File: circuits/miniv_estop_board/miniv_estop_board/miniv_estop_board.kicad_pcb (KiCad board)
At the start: 2 copper layers, 100 x 130 mm, 47 parts, among them J1 Conn_Main_DCDC, J2 Conn_neopixel_01, J3 Conn_neopixel_02, J4 Conn_neopixel_03, J5 Conn_neopixel_04, J6 EStop_button, J7 EStop_signal0, J8 EStop_signal1, Q1 2SJ555-E, Q2 NPN, Q3 NPN, Q4 NPN, Q6 2SJ555-E, Q7 NPN, U1 Teensy4.1

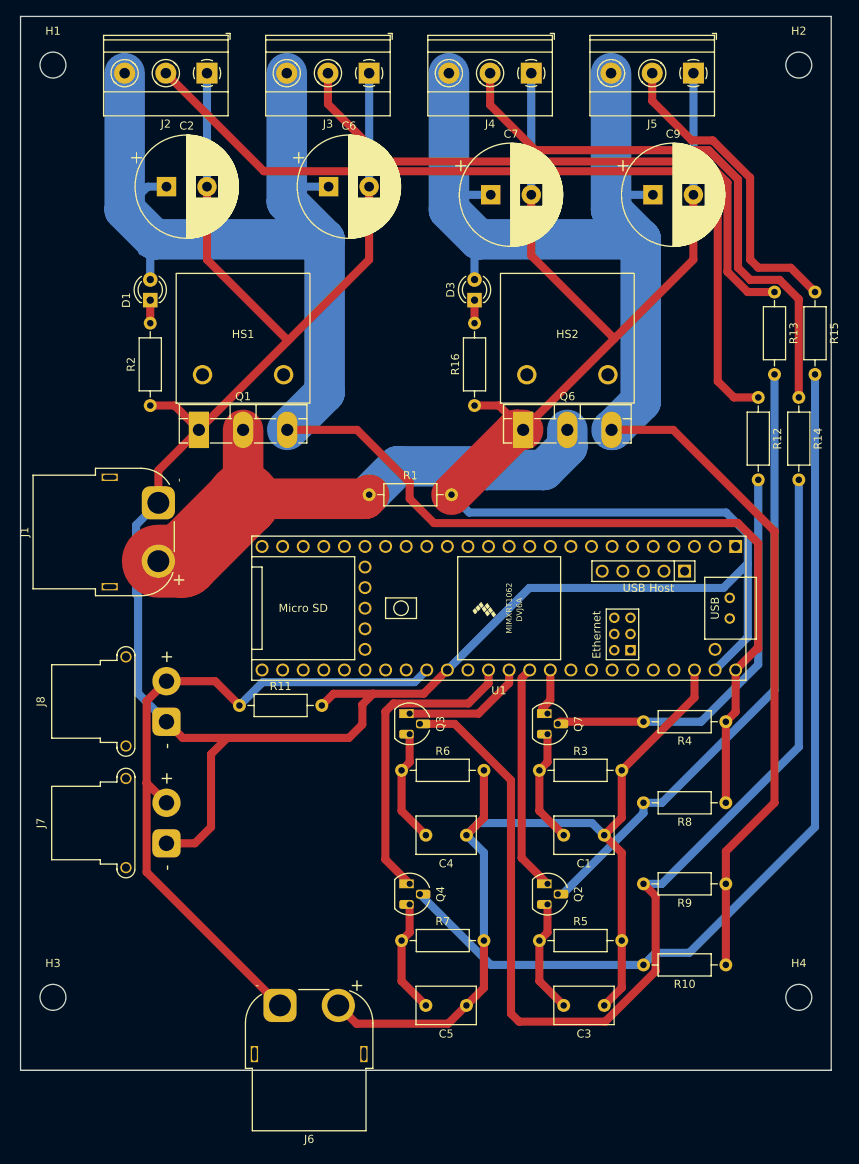
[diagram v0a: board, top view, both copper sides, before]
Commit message: update pcb
Signed-off-by: Masaya Kataoka <ms.kataoka@gmail.com>
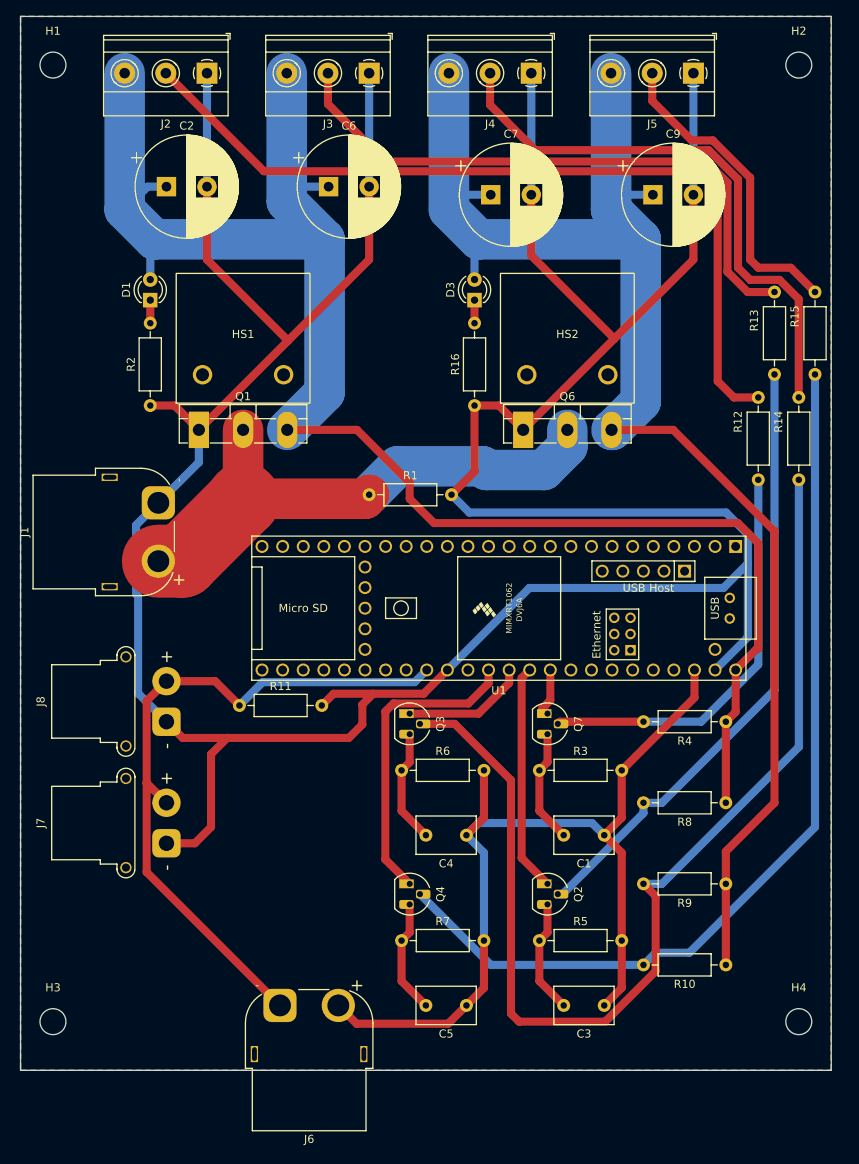
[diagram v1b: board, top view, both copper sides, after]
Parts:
- moved H3 3.00 mm to (96.0, 137.0)
- moved H4 3.00 mm to (188.0, 137.0)
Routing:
- net Net-(D1-A): track 209.2 -> 207.1 mm
- added copper zone on B.Cu, net GND
- added copper zone on F.Cu, net GND
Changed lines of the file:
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@@
 			(layer "F.Fab")
 		)
-		(fp_text user "-"
-			(at 2.8 2.5 90)
+		(fp_text user "+"
+			(at -9.5 2.5 90)
 			(layer "F.SilkS")
 			(effects
 				(font
-					(size 1 1)
+					(size 1.5 1.5)
 					(thickness 0.15)
 				)
 			)
 		)
-		(fp_text user "+"
-			(at -9.5 2.5 90)
+		(fp_text user "-"
+			(at 2.8 2.5 90)
 			(layer "F.SilkS")
 			(effects
 				(font
-					(size 1.5 1.5)
+					(size 1 1)
 					(thickness 0.15)
 				)
@@
 		(tags "Resistor Axial_DIN0207 series Axial Horizontal pin pitch 10.16mm 0.25W = 1/4W length 6.3mm diameter 2.5mm")
 		(property "Reference" "R13"
-			(at 5.08 -2.37 -90)
+			(at 3.5 2.5 -90)
 			(layer "F.SilkS")
 			(effects
@@
 		)
 		(property "Value" "470"
-			(at 5.08 2.37 -90)
+			(at 7 2.5 -90)
 			(layer "F.Fab")
 			(effects
@@
 		(tags "Resistor Axial_DIN0207 series Axial Horizontal pin pitch 10.16mm 0.25W = 1/4W length 6.3mm diameter 2.5mm")
 		(property "Reference" "R12"
-			(at 5.08 -2.37 -90)
+			(at 3 2.5 -90)
 			(layer "F.SilkS")
 			(effects
@@
 		)
 		(property "Value" "470"
-			(at 5.08 2.37 -90)
+			(at 7 2.37 -90)
 			(layer "F.Fab")
 			(effects
@@
 		(tags "LED diameter 3.0mm 2 pins")
 		(property "Reference" "D1"
-			(at 0 -2.96 90)
+			(at 1.27 -2.96 90)
 			(layer "F.SilkS")
 			(effects
@@
 		)
 		(property "Value" "LED"
-			(at 3 -3 90)
+			(at 1.27 2.96 90)
 			(layer "F.Fab")
 			(effects
@@
 		(tags "Resistor Axial_DIN0207 series Axial Horizontal pin pitch 10.16mm 0.25W = 1/4W length 6.3mm diameter 2.5mm")
 		(property "Reference" "R15"
-			(at 5.08 -2.37 -90)
+			(at 3 2.5 -90)
 			(layer "F.SilkS")
 			(effects
@@
 		)
 		(property "Value" "470"
-			(at 5.08 2.37 -90)
+			(at 6.5 2.5 -90)
 			(layer "F.Fab")
 			(effects
@@
 	(footprint "MountingHole:MountingHole_3.2mm_M3"
 		(layer "F.Cu")
-		(at 188 134)
+		(at 188 137)
 		(descr "Mounting Hole 3.2mm, no annular, M3")
 		(tags "mounting hole 3.2mm no annular m3")
@@
 			(layer "F.Fab")
 		)
-		(fp_text user "-"
-			(at -3 0 90)
+		(fp_text user "+"
+			(at 8 0 90)
 			(layer "F.SilkS")
 			(effects
@@
 			)
 		)
-		(fp_text user "+"
-			(at 8 0 90)
+		(fp_text user "-"
+			(at -3 0 90)
 			(layer "F.SilkS")
 			(effects
@@
 	(footprint "MountingHole:MountingHole_3.2mm_M3"
 		(layer "F.Cu")
-		(at 96 134)
+		(at 96 137)
 		(descr "Mounting Hole 3.2mm, no annular, M3")
 		(tags "mounting hole 3.2mm no annular m3")
@@
 		(tags "Resistor Axial_DIN0207 series Axial Horizontal pin pitch 10.16mm 0.25W = 1/4W length 6.3mm diameter 2.5mm")
 		(property "Reference" "R14"
-			(at 5.08 -2.37 -90)
+			(at 3 2.5 -90)
 			(layer "F.SilkS")
 			(effects
@@
 		)
 		(property "Value" "470"
-			(at 5.08 2.37 -90)
+			(at 7 2.37 -90)
 			(layer "F.Fab")
 			(effects
@@
 		)
 		(property "Value" "MountingHole"
-			(at 0 4.2 0)
+			(at -3 4.5 0)
 			(layer "F.Fab")
 			(effects
@@
 		)
 		(property "Value" "MountingHole"
-			(at 2.5 4.5 0)
+			(at 4 6.5 90)
 			(layer "F.Fab")
 			(effects
@@
 			(layer "F.Fab")
 		)
-		(fp_text user "-"
-			(at 2.8 2.5 180)
+		(fp_text user "+"
+			(at -9.5 2.5 180)
 			(layer "F.SilkS")
 			(effects
 				(font
-					(size 1 1)
+					(size 1.5 1.5)
 					(thickness 0.15)
 				)
 			)
 		)
-		(fp_text user "+"
-			(at -9.5 2.5 180)
+		(fp_text user "-"
+			(at 2.8 2.5 180)
 			(layer "F.SilkS")
 			(effects
 				(font
-					(size 1.5 1.5)
+					(size 1 1)
 					(thickness 0.15)
 				)
@@
 	)
 	(segment
-		(start 107 42.001523)
-		(end 108.501523 40.5)
-		(width 1)
-		(layer "B.Cu")
-		(net 6)
-	)
-	(segment
 		(start 130 34)
 		(end 126.68 34)
@@
 	)
 	(segment
-		(start 153.16 64)
-		(end 145.16 72)
-		(width 5)
-		(layer "F.Cu")
-		(net 11)
-	)
-	(segment
 		(start 129.16 98)
 		(end 130.61 96.55)
@@
 	)
 	(segment
-		(start 109 73)
-		(end 109 69)
+		(start 175 43)
+		(end 175 35)
 		(width 1)
 		(layer "F.Cu")
@@
 	)
 	(segment
-		(start 175 43)
-		(end 175 35)
+		(start 148 69.16)
+		(end 145.16 72)
 		(width 1)
 		(layer "F.Cu")
@@
 	)
 	(segment
-		(start 109 69)
-		(end 114 64)
-		(width 1)
-		(layer "F.Cu")
-		(net 11)
-	)
-	(segment
 		(start 155 42.5)
 		(end 155 35)
@@
 	)
 	(segment
-		(start 154 64)
-		(end 153.16 64)
-		(width 5)
-		(layer "F.Cu")
-		(net 11)
-	)
-	(segment
 		(start 165.25 52.75)
 		(end 155 42.5)
@@
 	)
 	(segment
+		(start 148 61)
+		(end 148 69.16)
+		(width 1)
+		(layer "F.Cu")
+		(net 11)
+	)
+	(segment
 		(start 165.25 52.75)
 		(end 154 64)
@@
 	)
 	(segment
+		(start 114 64)
+		(end 114 68)
+		(width 1)
+		(layer "B.Cu")
+		(net 11)
+	)
+	(segment
 		(start 181.71 80.5)
 		(end 181.71 89.58)
@@
 	)
 	(segment
+		(start 114 68)
+		(end 109 73)
+		(width 1)
+		(layer "B.Cu")
+		(net 11)
+	)
+	(segment
 		(start 106.25 75.75)
 		(end 106.25 84.25)
@@
 		(net 82)
 	)
+	(zone
+		(net 11)
+		(net_name "GND")
+		(layers "F&B.Cu")
+		(hatch edge 0.5)
+		(connect_pads
+			(clearance 0.5)
+		)
+		(min_thickness 0.25)
+		(filled_areas_thickness no)
+		(fill yes
+			(thermal_gap 0.5)
+			(thermal_bridge_width 0.5)
+		)
+		(polygon
+			(pts
+				(xy 192 13) (xy 92 13) (xy 92 143) (xy 192 143)
+			)
+		)
+	)
 )
